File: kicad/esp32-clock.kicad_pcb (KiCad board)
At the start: 2 copper layers, 37 x 40 mm, 36 parts, among them J1 Conn_01x07_Socket, P1 USB_C_Plug_USB2.0, Q1 BCW66G, Q2 BCW66G, SW1 RESET, SW2 BOOT, U1 ESP32-PICO-V3, U2 USBLC6-2P6, U3 AMS1117-3.3, U4 CP2102N-Axx-xQFN28

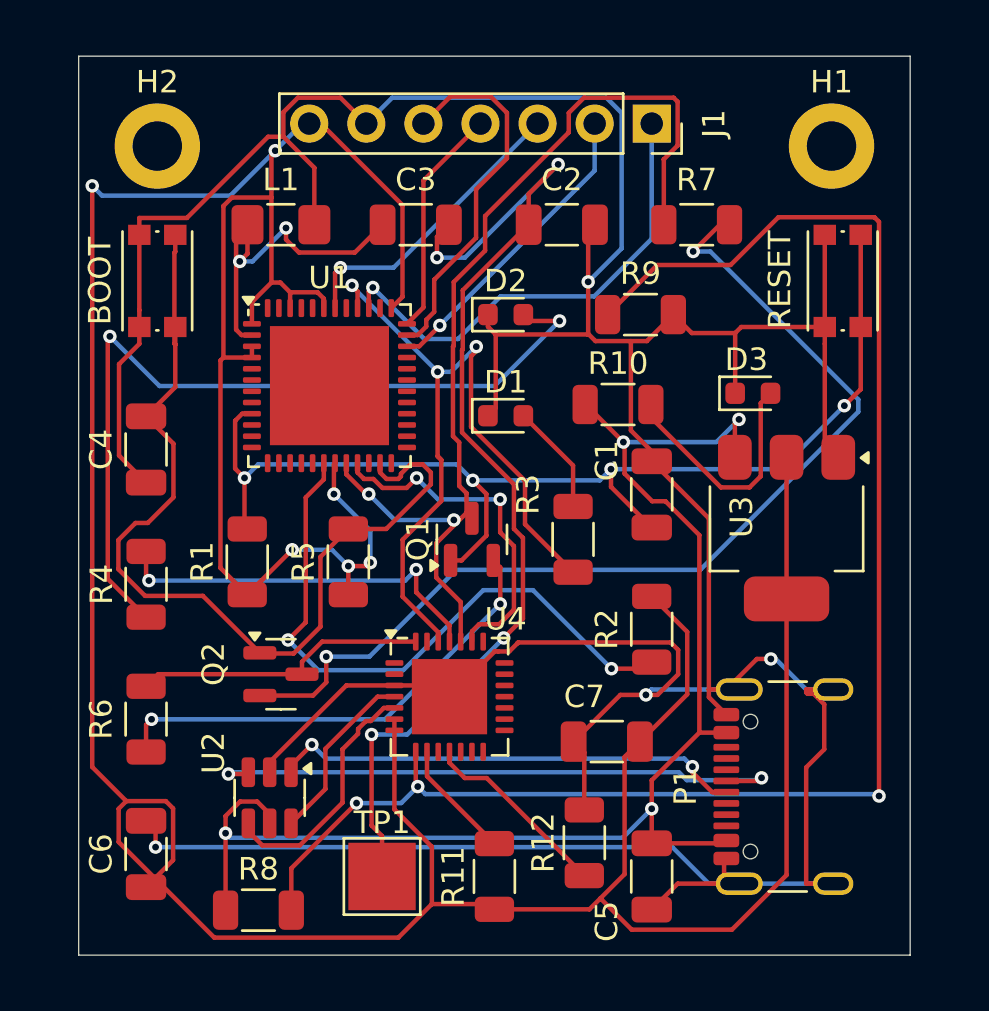
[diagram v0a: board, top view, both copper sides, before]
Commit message: init
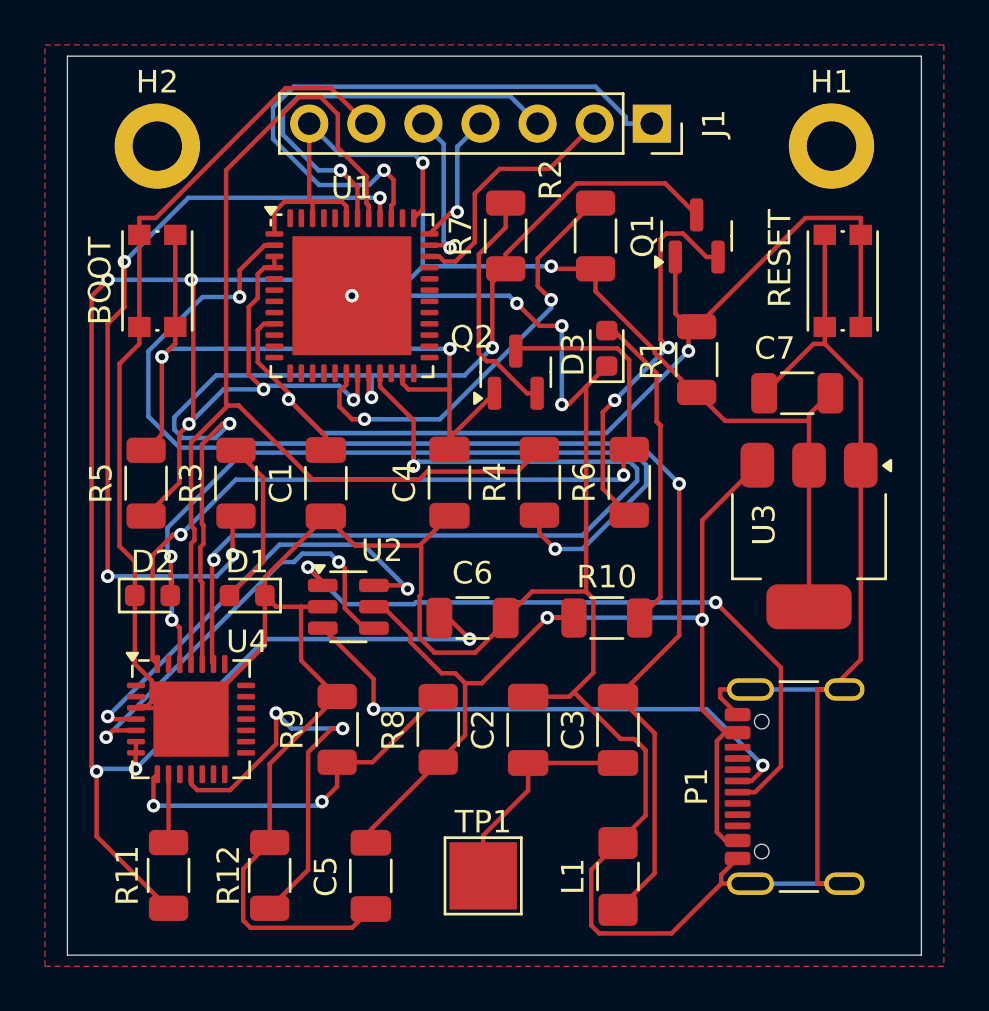
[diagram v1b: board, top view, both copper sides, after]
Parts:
- moved L1 32.6 mm to (143.0, 93.0), turned to 90 degrees
- moved C3 24.2 mm to (143.0, 86.5), turned to 90 degrees
- moved R6 23.9 mm to (143.5, 75.5)
- moved R9 22.9 mm to (130.5, 86.5), turned to 90 degrees
- moved C2 22.5 mm to (139.0, 86.5), turned to 90 degrees
- moved R1 21.9 mm to (146.5, 70.0)
- moved D2 20.1 mm to (122.3, 80.5)
- moved R4 18.1 mm to (139.5, 75.5)
- moved C6 17.9 mm to (136.5, 81.5), turned to 0 degrees
- moved R2 17.7 mm to (142.0, 64.5), turned to -90 degrees
- moved C7 17.7 mm to (151.0, 71.5)
- moved Q2 17.0 mm to (138.4, 70.6), turned to 90 degrees
- moved Q1 16.8 mm to (146.5, 64.5)
- moved R3 15.2 mm to (126.0, 75.5)
- moved C1 14.5 mm to (130.0, 75.5), turned to -90 degrees
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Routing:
- net Net-(U4-VBUS): track 70.8 -> 16.8 mm, vias 3 -> 2
- net Net-(U1-LNA_IN): track 15.7 -> 57.6 mm
- net Net-(C2-Pad1): track 48.0 -> 9.85 mm, vias 4 -> 0
- net +3.3V: track 181.8 -> 146.6 mm, vias 6 -> 10
- net Net-(Q2-B): track 45.3 -> 10.5 mm, vias 2 -> 0
- net /supply/RXD: track 17.3 -> 50.4 mm, vias 2 -> 0
- net /CTS: track 15.5 -> 40.6 mm
- net /supply/DTR: track 13.1 -> 37.9 mm, vias 0 -> 2
- net +5V: track 61.4 -> 47.0 mm, vias 4 -> 2
- net Net-(U4-D+): track 7.98 -> 20.2 mm, vias 0 -> 2
- net Net-(U4-~{SUSPEND}): track 8.57 -> 19.4 mm, vias 0 -> 2
- net Net-(P1-D+): track 21.1 -> 30.8 mm
- net Net-(J1-Pin_5): track 16.5 -> 6.98 mm, vias 0 -> 1
- net /IO0: track 42.3 -> 33.3 mm, vias 0 -> 2
- net Net-(U1-IO12): track 28.3 -> 19.4 mm
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- added copper zone on F.Cu, net GND
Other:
- board size 37 x 40 mm -> 38 x 40 mm
